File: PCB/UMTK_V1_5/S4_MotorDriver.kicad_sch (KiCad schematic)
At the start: 17 parts, among them J1 Motor Out, J2 ESTOP, U1 DRV8873SPWPRQ1

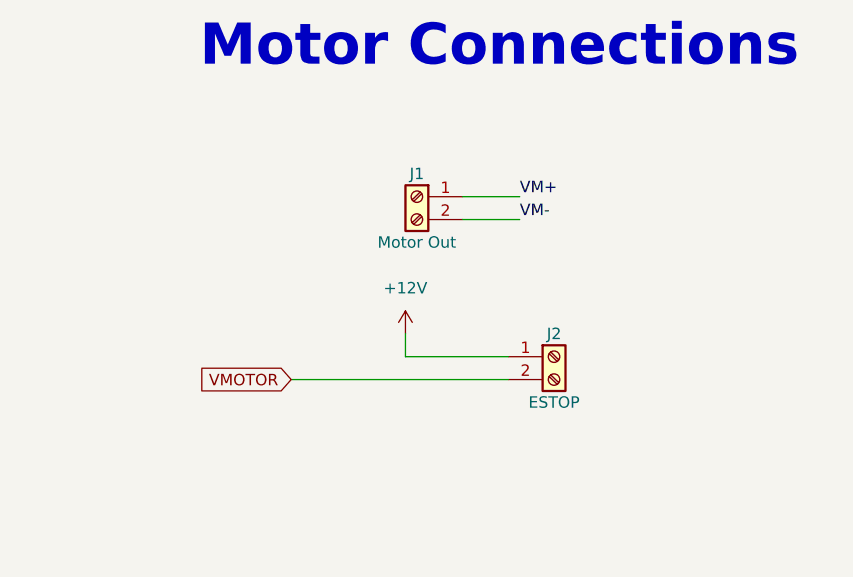
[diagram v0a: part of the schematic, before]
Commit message: Routing
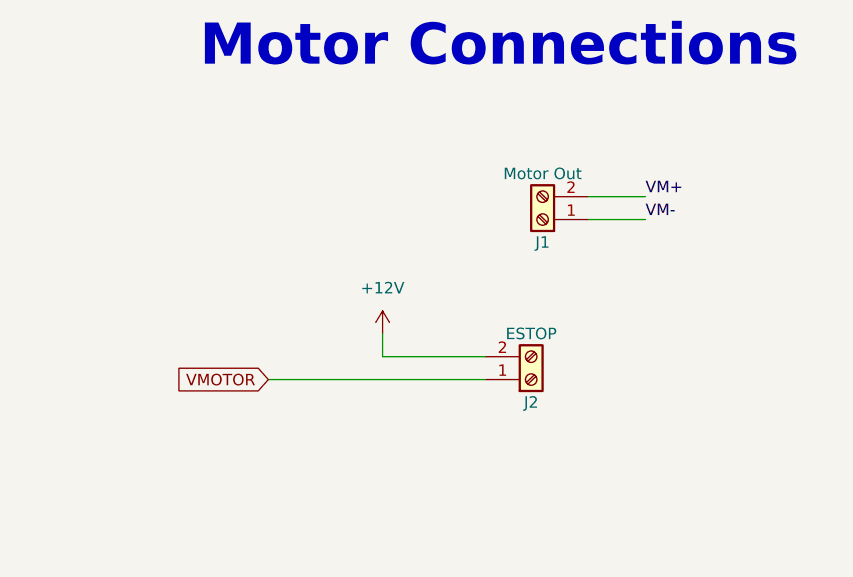
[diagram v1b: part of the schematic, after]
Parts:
- J1, J2: footprint TerminalBlock_Altech:Altech_AK100_1x02_P5.00mm -> Connector_Phoenix_MC_HighVoltage:PhoenixContact_MC_1,5_2-G-5.08_1x02_P5.08mm_Horizontal
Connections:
- net +12V: now also J2.2 (Pin_2); no longer J2.1 (Pin_1)
- net VM+: now also J1.2 (Pin_2); no longer J1.1 (Pin_1)
- net VM-: now also J1.1 (Pin_1); no longer J1.2 (Pin_2)
- net VMOTOR: now also J2.1 (Pin_1); no longer J2.2 (Pin_2)
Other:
- moved on the sheet: J1, J2
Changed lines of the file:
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@@
-	(wire
-		(pts
-			(xy 233.68 67.31) (xy 233.68 69.85)
-		)
-		(stroke
-			(width 0)
-			(type default)
-		)
-	)
 	(wire
 		(pts
@@
 	(wire
 		(pts
+			(xy 231.14 69.85) (xy 242.57 69.85)
+		)
+		(stroke
+			(width 0)
+			(type default)
+		)
+	)
+	(wire
+		(pts
 			(xy 113.03 156.21) (xy 113.03 148.59)
 		)
@@
 	(wire
 		(pts
-			(xy 220.98 72.39) (xy 245.11 72.39)
-		)
-		(stroke
-			(width 0)
-			(type default)
-		)
-	)
-	(wire
-		(pts
 			(xy 97.79 153.67) (xy 97.79 156.21)
 		)
@@
 	(wire
 		(pts
-			(xy 240.03 52.07) (xy 246.38 52.07)
-		)
-		(stroke
-			(width 0)
-			(type default)
-		)
-	)
-	(wire
-		(pts
 			(xy 81.28 140.97) (xy 93.98 140.97)
 		)
@@
 	(wire
 		(pts
-			(xy 233.68 69.85) (xy 245.11 69.85)
-		)
-		(stroke
-			(width 0)
-			(type default)
-		)
-	)
-	(wire
-		(pts
 			(xy 81.28 146.05) (xy 81.28 154.94)
 		)
@@
 	(wire
 		(pts
+			(xy 254 54.61) (xy 260.35 54.61)
+		)
+		(stroke
+			(width 0)
+			(type default)
+		)
+	)
+	(wire
+		(pts
 			(xy 182.88 161.29) (xy 182.88 163.83)
 		)
@@
 	(wire
 		(pts
-			(xy 240.03 54.61) (xy 246.38 54.61)
+			(xy 218.44 72.39) (xy 242.57 72.39)
 		)
 		(stroke
@@
 	(wire
 		(pts
+			(xy 231.14 67.31) (xy 231.14 69.85)
+		)
+		(stroke
+			(width 0)
+			(type default)
+		)
+	)
+	(wire
+		(pts
 			(xy 173.99 146.05) (xy 180.34 146.05)
 		)
@@
 		(pts
 			(xy 81.28 146.05) (xy 138.43 146.05)
+		)
+		(stroke
+			(width 0)
+			(type default)
+		)
+	)
+	(wire
+		(pts
+			(xy 254 52.07) (xy 260.35 52.07)
 		)
 		(stroke
@@
 		)
 	)
-	(label "VM-"
-		(at 246.38 54.61 0)
+	(label "SR - Slew Rate Adjust"
+		(at 85.09 146.05 0)
 		(fields_autoplaced yes)
 		(effects
@@
 		)
 	)
-	(label "SR - Slew Rate Adjust"
-		(at 85.09 146.05 0)
+	(label "VM+"
+		(at 181.61 128.27 0)
 		(fields_autoplaced yes)
 		(effects
@@
 	)
 	(label "VM+"
-		(at 181.61 128.27 0)
+		(at 260.35 52.07 0)
 		(fields_autoplaced yes)
 		(effects
@@
 		)
 	)
-	(label "VM+"
-		(at 246.38 52.07 0)
+	(label "VM-"
+		(at 260.35 54.61 0)
 		(fields_autoplaced yes)
 		(effects
@@
 	(global_label "VMOTOR"
 		(shape input)
-		(at 220.98 72.39 180)
+		(at 215.9 110.49 180)
 		(fields_autoplaced yes)
 		(effects
@@
 		)
 		(property "Intersheetrefs" "${INTERSHEET_REFS}"
-			(at 210.5562 72.39 0)
+			(at 205.4762 110.49 0)
 			(effects
 				(font
@@
 	(global_label "VMOTOR"
 		(shape input)
-		(at 215.9 110.49 180)
+		(at 218.44 72.39 180)
 		(fields_autoplaced yes)
 		(effects
@@
 		)
 		(property "Intersheetrefs" "${INTERSHEET_REFS}"
-			(at 205.4762 110.49 0)
+			(at 208.0162 72.39 0)
 			(effects
 				(font
@@
 	)
 	(symbol
+		(lib_id "power:+12V")
+		(at 231.14 67.31 0)
+		(unit 1)
+		(exclude_from_sim no)
+		(in_bom yes)
+		(on_board yes)
+		(dnp no)
+		(fields_autoplaced yes)
+		(property "Reference" "#PWR07"
+			(at 231.14 71.12 0)
+			(effects
+				(font
+					(size 1.27 1.27)
+				)
+				(hide yes)
+			)
+		)
+		(property "Value" "+12V"
+			(at 231.14 62.23 0)
+			(effects
+				(font
+					(size 1.27 1.27)
+				)
+			)
+		)
+		(property "Footprint" ""
+			(at 231.14 67.31 0)
+			(effects
+				(font
+					(size 1.27 1.27)
+				)
+				(hide yes)
+			)
+		)
+		(property "Datasheet" ""
+			(at 231.14 67.31 0)
+			(effects
+				(font
+					(size 1.27 1.27)
+				)
+				(hide yes)
+			)
+		)
+		(property "Description" "Power symbol creates a global label with name \"+12V\""
+			(at 231.14 67.31 0)
+			(effects
+				(font
+					(size 1.27 1.27)
+				)
+				(hide yes)
+			)
+		)
+		(pin "1"
+		)
+		(instances
+			(project "UMTK"
+				(path "/2bf3ea67-58b8-47b3-a768-ea6950b40edf/429db1c7-ec58-4147-903c-f97ceea1f1c2"
+					(reference "#PWR07")
+					(unit 1)
+				)
+			)
+		)
+	)
+	(symbol
 		(lib_id "power:GND")
 		(at 199.39 156.21 0)
@@
 	(symbol
 		(lib_id "Connector:Screw_Terminal_01x02")
-		(at 234.95 52.07 0)
-		(mirror y)
+		(at 248.92 54.61 180)
 		(unit 1)
 		(exclude_from_sim no)
@@
 		(dnp no)
 		(property "Reference" "J1"
-			(at 234.95 49.53 0)
+			(at 248.92 57.15 0)
 			(effects
 				(font
@@
 		)
 		(property "Value" "Motor Out"
-			(at 234.95 57.15 0)
-			(effects
-				(font
-					(size 1.27 1.27)
-				)
-			)
-		)
-		(property "Footprint" "TerminalBlock_Altech:Altech_AK100_1x02_P5.00mm"
-			(at 234.95 52.07 0)
+			(at 248.92 49.53 0)
+			(effects
+				(font
+					(size 1.27 1.27)
+				)
+			)
+		)
+		(property "Footprint" "Connector_Phoenix_MC_HighVoltage:PhoenixContact_MC_1,5_2-G-5.08_1x02_P5.08mm_Horizontal"
+			(at 248.92 54.61 0)
 			(effects
 				(font
@@
 		)
 		(property "Datasheet" "~"
-			(at 234.95 52.07 0)
+			(at 248.92 54.61 0)
 			(effects
 				(font
@@
 		)
 		(property "Description" "Generic screw terminal, single row, 01x02, script generated (kicad-library-utils/schlib/autogen/connector/)"
-			(at 234.95 52.07 0)
+			(at 248.92 54.61 0)
 			(effects
 				(font
@@
 	)
 	(symbol
-		(lib_id "power:+12V")
-		(at 233.68 67.31 0)
-		(unit 1)
-		(exclude_from_sim no)
-		(in_bom yes)
-		(on_board yes)
-		(dnp no)
-		(fields_autoplaced yes)
-		(property "Reference" "#PWR018"
-			(at 233.68 71.12 0)
-			(effects
-				(font
-					(size 1.27 1.27)
-				)
-				(hide yes)
-			)
-		)
-		(property "Value" "+12V"
-			(at 233.68 62.23 0)
-			(effects
-				(font
-					(size 1.27 1.27)
-				)
-			)
-		)
-		(property "Footprint" ""
-			(at 233.68 67.31 0)
-			(effects
-				(font
-					(size 1.27 1.27)
-				)
-				(hide yes)
-			)
-		)
-		(property "Datasheet" ""
-			(at 233.68 67.31 0)
-			(effects
-				(font
-					(size 1.27 1.27)
-				)
-				(hide yes)
-			)
-		)
-		(property "Description" "Power symbol creates a global label with name \"+12V\""
-			(at 233.68 67.31 0)
-			(effects
-				(font
-					(size 1.27 1.27)
-				)
-				(hide yes)
-			)
-		)
-		(pin "1"
-		)
-		(instances
-			(project ""
-				(path "/2bf3ea67-58b8-47b3-a768-ea6950b40edf/429db1c7-ec58-4147-903c-f97ceea1f1c2"
-					(reference "#PWR018")
-					(unit 1)
-				)
-			)
-		)
-	)
-	(symbol
 		(lib_id "Device:C")
 		(at 201.93 127 180)
@@
 	(symbol
 		(lib_id "Connector:Screw_Terminal_01x02")
-		(at 250.19 69.85 0)
+		(at 247.65 72.39 0)
+		(mirror x)
 		(unit 1)
 		(exclude_from_sim no)
@@
 		(dnp no)
 		(property "Reference" "J2"
-			(at 250.19 67.31 0)
+			(at 247.65 74.93 0)
 			(effects
 				(font
@@
 		)
 		(property "Value" "ESTOP"
-			(at 250.19 74.93 0)
-			(effects
-				(font
-					(size 1.27 1.27)
-				)
-			)
-		)
-		(property "Footprint" "TerminalBlock_Altech:Altech_AK100_1x02_P5.00mm"
-			(at 250.19 69.85 0)
+			(at 247.65 67.31 0)
+			(effects
+				(font
+					(size 1.27 1.27)
+				)
+			)
+		)
+		(property "Footprint" "Connector_Phoenix_MC_HighVoltage:PhoenixContact_MC_1,5_2-G-5.08_1x02_P5.08mm_Horizontal"
+			(at 247.65 72.39 0)
 			(effects
 				(font
@@
 		)
 		(property "Datasheet" "~"
-			(at 250.19 69.85 0)
+			(at 247.65 72.39 0)
 			(effects
 				(font
@@
 		)
 		(property "Description" "Generic screw terminal, single row, 01x02, script generated (kicad-library-utils/schlib/autogen/connector/)"
-			(at 250.19 69.85 0)
-			(effects
-				(font
+			(at 247.65 72.39 0)
+			(effects
+				(font
